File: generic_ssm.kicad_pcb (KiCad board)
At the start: 4 copper layers, 80 x 80 mm, 20 parts, among them J1 RST_JMP, J2 DEBUG CONN, J3 PROGRAMMING PORT, SW1 SW_RST, U1 SN65HVD233, U2 ATMEGA32M1-MU, Y1 8MHz

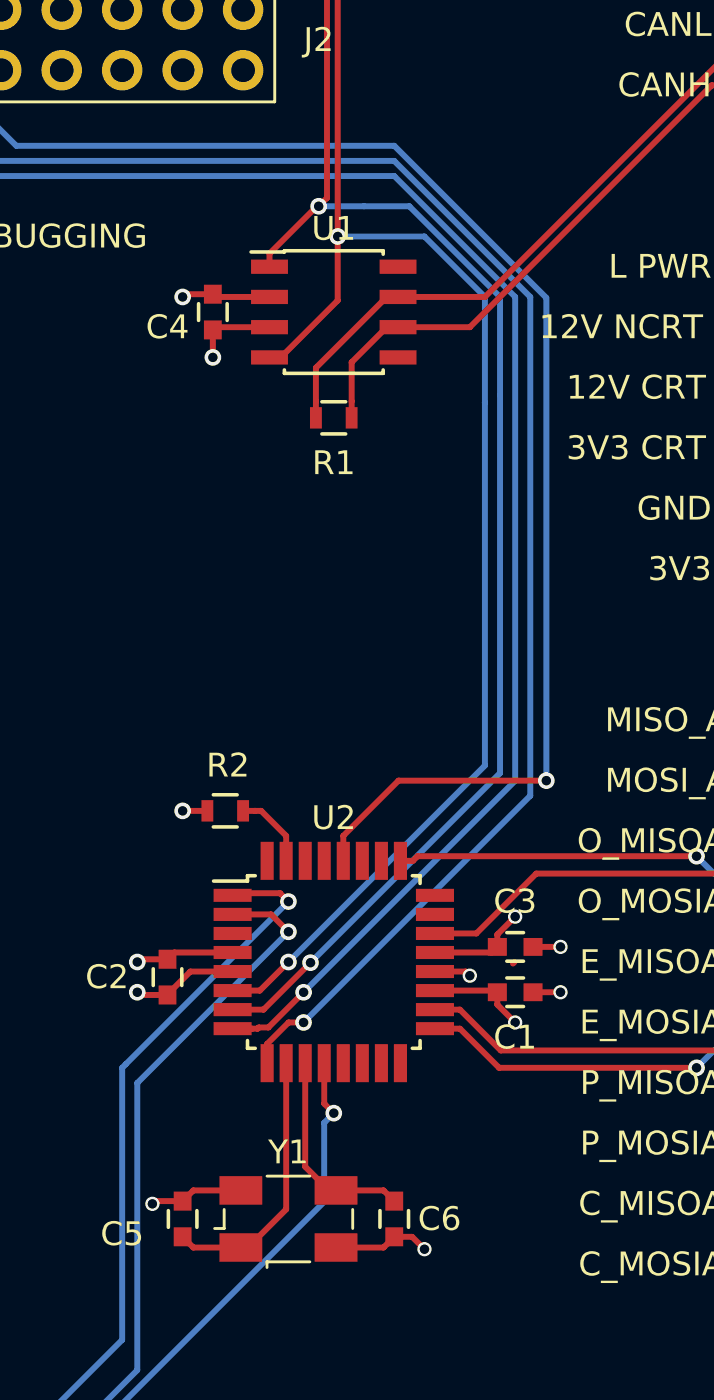
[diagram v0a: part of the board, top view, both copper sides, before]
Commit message: Minor Changes
Fixed via sizes, fixed resistors on schematic
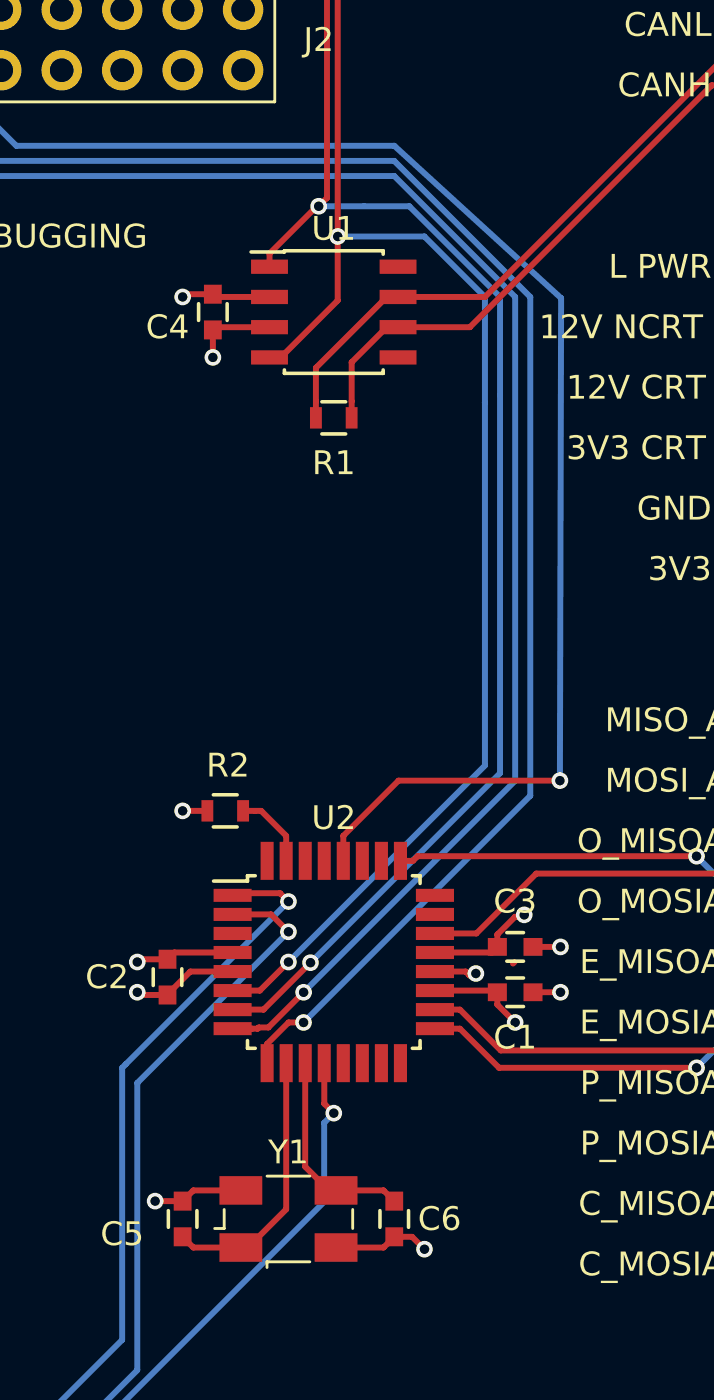
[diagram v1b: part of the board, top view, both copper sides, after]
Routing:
- net /SCK: track 60.2 -> 61.2 mm
- net GND: track 30.9 -> 31.5 mm
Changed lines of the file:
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@@
     (links 64)
     (no_connects 19)
-    (area 99.924999 49.924999 180.075001 130.075001)
+    (area 99.924999 46.723 218.11224 130.075001)
     (thickness 1.6)
     (drawings 56)
-    (tracks 271)
+    (tracks 280)
     (zones 0)
     (modules 20)
@@
     (aux_axis_origin 0 0)
     (grid_origin 12.192 12.573)
-    (visible_elements FFFEFF7F)
+    (visible_elements 7FFFFFFF)
     (pcbplotparams
       (layerselection 0x00030_80000001)
@@
   (gr_line (start 100 50) (end 180 50) (angle 90) (layer Edge.Cuts) (width 0.15))
   (segment (start 159.422001 95.823001) (end 159.487001 95.758001) (width 0.25) (layer F.Cu) (net 0))
+  (segment (start 157.5862 96.3122) (end 157.7894 96.3122) (width 0.25) (layer F.Cu) (net 1))
+  (via (at 157.861 96.2406) (size 0.7) (drill 0.4) (layers F.Cu B.Cu) (net 1))
+  (segment (start 157.7894 96.3122) (end 157.861 96.2406) (width 0.25) (layer F.Cu) (net 1))
+  (via (at 155.702 107.823) (size 0.7) (drill 0.4) (layers F.Cu B.Cu) (net 1))
+  (segment (start 144.272 105.918) (end 144.387 105.803) (width 0.25) (layer F.Cu) (net 1))
+  (segment (start 144.387 105.803) (end 144.272 105.918) (width 0.25) (layer F.Cu) (net 1))
+  (via (at 144.387 105.803) (size 0.7) (drill 0.4) (layers F.Cu B.Cu) (net 1))
+  (segment (start 144.387 105.803) (end 144.3736 105.8164) (width 0.25) (layer B.Cu) (net 1))
+  (segment (start 144.3736 105.8164) (end 144.3228 105.8164) (width 0.25) (layer B.Cu) (net 1))
   (segment (start 149.822 124.678) (end 153.452 124.678) (width 0.25) (layer F.Cu) (net 1))
   (segment (start 153.452 124.678) (end 153.797 124.333) (width 0.25) (layer F.Cu) (net 1))
@@
   (segment (start 157.772 124.678) (end 158.587 124.678) (width 0.25) (layer F.Cu) (net 1))
   (segment (start 156.142 96.158) (end 157.432 96.158) (width 0.25) (layer F.Cu) (net 1))
-  (via (at 157.607 96.333) (size 0.6) (drill 0.4) (layers F.Cu B.Cu) (net 1))
-  (segment (start 157.432 96.158) (end 157.607 96.333) (width 0.25) (layer F.Cu) (net 1))
+  (segment (start 157.432 96.158) (end 157.5862 96.3122) (width 0.25) (layer F.Cu) (net 1))
+  (segment (start 157.5862 96.3122) (end 157.607 96.333) (width 0.25) (layer F.Cu) (net 1))
   (segment (start 160.262 97.028) (end 161.417 97.028) (width 0.25) (layer F.Cu) (net 1))
-  (via (at 161.417 97.028) (size 0.6) (drill 0.4) (layers F.Cu B.Cu) (net 1))
+  (via (at 161.417 97.028) (size 0.7) (drill 0.4) (layers F.Cu B.Cu) (net 1))
   (segment (start 160.262 95.123) (end 161.417 95.123) (width 0.25) (layer F.Cu) (net 1))
-  (via (at 161.417 95.123) (size 0.6) (drill 0.4) (layers F.Cu B.Cu) (net 1))
+  (via (at 161.417 95.123) (size 0.7) (drill 0.4) (layers F.Cu B.Cu) (net 1))
   (segment (start 145.542 105.803) (end 144.387 105.803) (width 0.25) (layer F.Cu) (net 1))
-  (segment (start 144.387 105.803) (end 144.272 105.918) (width 0.25) (layer F.Cu) (net 1))
-  (via (at 144.272 105.918) (size 0.6) (drill 0.4) (layers F.Cu B.Cu) (net 1))
   (segment (start 147.987 105.353) (end 145.992 105.353) (width 0.25) (layer F.Cu) (net 1))
   (segment (start 145.992 105.353) (end 145.542 105.803) (width 0.25) (layer F.Cu) (net 1))
   (segment (start 154.432 107.303) (end 155.182 107.303) (width 0.25) (layer F.Cu) (net 1))
   (segment (start 155.182 107.303) (end 155.702 107.823) (width 0.25) (layer F.Cu) (net 1))
-  (via (at 155.702 107.823) (size 0.6) (drill 0.4) (layers F.Cu B.Cu) (net 1))
   (segment (start 151.987 107.753) (end 153.982 107.753) (width 0.25) (layer F.Cu) (net 1))
   (segment (start 153.982 107.753) (end 154.432 107.303) (width 0.25) (layer F.Cu) (net 1))
+  (segment (start 159.4993 93.8657) (end 159.8041 93.8657) (width 0.25) (layer F.Cu) (net 2))
+  (via (at 159.893 93.7768) (size 0.7) (drill 0.4) (layers F.Cu B.Cu) (net 2))
+  (segment (start 159.8041 93.8657) (end 159.893 93.7768) (width 0.25) (layer F.Cu) (net 2))
   (segment (start 146.582 89.408) (end 145.542 89.408) (width 0.25) (layer F.Cu) (net 2))
   (via (at 145.542 89.408) (size 0.7) (drill 0.4) (layers F.Cu B.Cu) (net 2))
@@
   (via (at 120.142 118.618) (size 0.7) (drill 0.4) (layers F.Cu B.Cu) (net 2))
   (segment (start 158.762 95.123) (end 158.762 94.603) (width 0.25) (layer F.Cu) (net 2))
-  (segment (start 158.762 94.603) (end 159.512 93.853) (width 0.25) (layer F.Cu) (net 2))
-  (via (at 159.512 93.853) (size 0.6) (drill 0.4) (layers F.Cu B.Cu) (net 2))
+  (segment (start 158.762 94.603) (end 159.4993 93.8657) (width 0.25) (layer F.Cu) (net 2))
+  (segment (start 159.4993 93.8657) (end 159.512 93.853) (width 0.25) (layer F.Cu) (net 2))
   (segment (start 156.142 95.358) (end 158.527 95.358) (width 0.25) (layer F.Cu) (net 2))
   (segment (start 158.527 95.358) (end 158.762 95.123) (width 0.25) (layer F.Cu) (net 2))
   (segment (start 158.762 97.028) (end 158.762 97.548) (width 0.25) (layer F.Cu) (net 2))
   (segment (start 158.762 97.548) (end 159.512 98.298) (width 0.25) (layer F.Cu) (net 2))
-  (via (at 159.512 98.298) (size 0.6) (drill 0.4) (layers F.Cu B.Cu) (net 2))
+  (via (at 159.512 98.298) (size 0.7) (drill 0.4) (layers F.Cu B.Cu) (net 2))
   (segment (start 156.142 96.958) (end 158.692 96.958) (width 0.25) (layer F.Cu) (net 2))
   (segment (start 158.692 96.958) (end 158.762 97.028) (width 0.25) (layer F.Cu) (net 2))
@@
   (segment (start 149.9926 98.298) (end 150.622 98.298) (width 0.25) (layer F.Cu) (net 49))
   (via (at 150.622 98.298) (size 0.7) (drill 0.4) (layers F.Cu B.Cu) (net 49))
-  (segment (start 160.822 88.138) (end 160.822 67.85518) (width 0.25) (layer B.Cu) (net 50))
-  (segment (start 160.822 67.85518) (end 154.43482 61.468) (width 0.25) (layer B.Cu) (net 50))
+  (segment (start 161.3916 88.138) (end 161.4424 67.8688) (width 0.25) (layer B.Cu) (net 50))
+  (segment (start 161.4424 67.8688) (end 154.43482 61.468) (width 0.25) (layer B.Cu) (net 50))
   (segment (start 154.43482 61.468) (end 138.557 61.468) (width 0.25) (layer B.Cu) (net 50))
   (segment (start 138.557 61.468) (end 135.382 58.293) (width 0.25) (layer B.Cu) (net 50))
   (segment (start 152.292 91.508) (end 152.292 90.458) (width 0.25) (layer F.Cu) (net 50))
   (segment (start 152.292 90.458) (end 154.612 88.138) (width 0.25) (layer F.Cu) (net 50))
-  (segment (start 154.612 88.138) (end 160.822 88.138) (width 0.25) (layer F.Cu) (net 50))
-  (via (at 160.822 88.138) (size 0.7) (drill 0.4) (layers F.Cu B.Cu) (net 50))
+  (segment (start 154.612 88.138) (end 161.3916 88.138) (width 0.25) (layer F.Cu) (net 50))
+  (via (at 161.3916 88.138) (size 0.7) (drill 0.4) (layers F.Cu B.Cu) (net 50))
   (segment (start 154.592 69.088) (end 157.60841 69.088) (width 0.25) (layer F.Cu) (net 60))
   (segment (start 157.60841 69.088) (end 167.76841 58.928) (width 0.25) (layer F.Cu) (net 60))
